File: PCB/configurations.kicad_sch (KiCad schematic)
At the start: 23 parts, among them SW1 SW_Push, U1 XC7A50T-FGG484, U7 MT25QL128ABA1EW7-0SIT

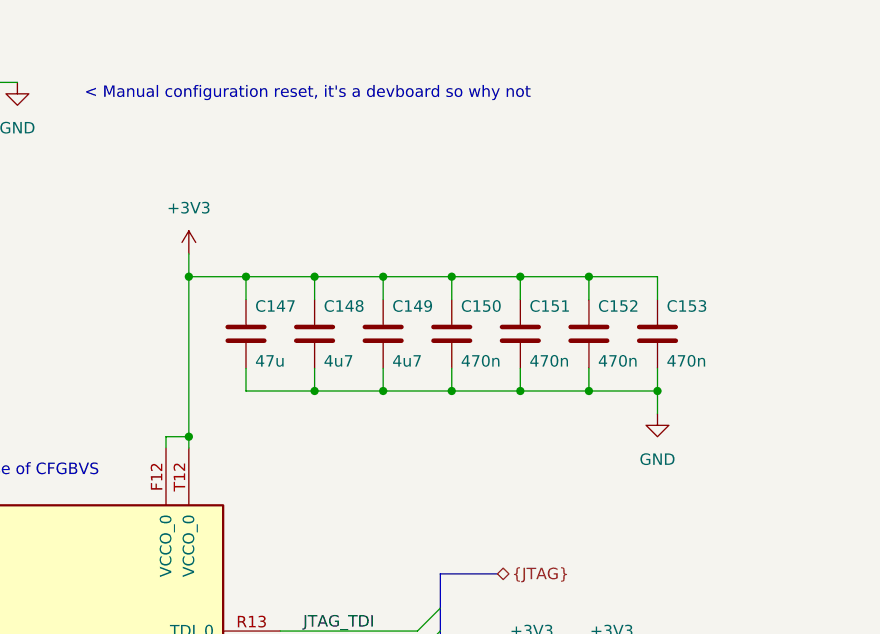
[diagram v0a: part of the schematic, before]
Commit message: fixed my decoupling because I'm better than the datasheet
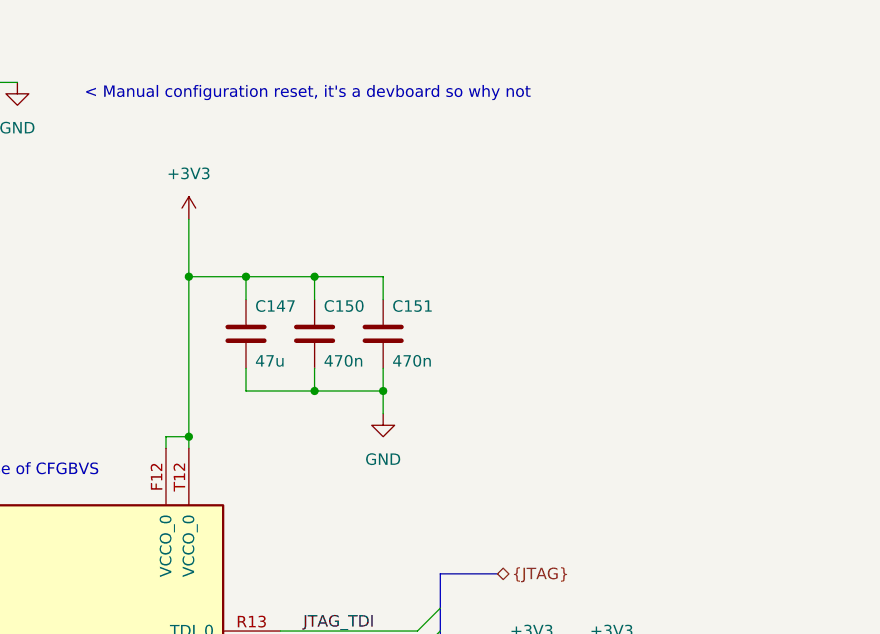
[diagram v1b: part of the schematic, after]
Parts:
- removed C148, C149: 4u7, Capacitor_SMD:C_0603_1608Metric, symbol Device:C
- removed C152, C153: 470n, Capacitor_SMD:C_0201_0603Metric, symbol Device:C
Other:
- moved on the sheet: C150, C151
